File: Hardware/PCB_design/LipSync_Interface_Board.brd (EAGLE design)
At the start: 69.8 x 63.5 mm, 31 parts, among them T1 2N3906, U2 SF_MATE_RN42, U3 MPXV7002

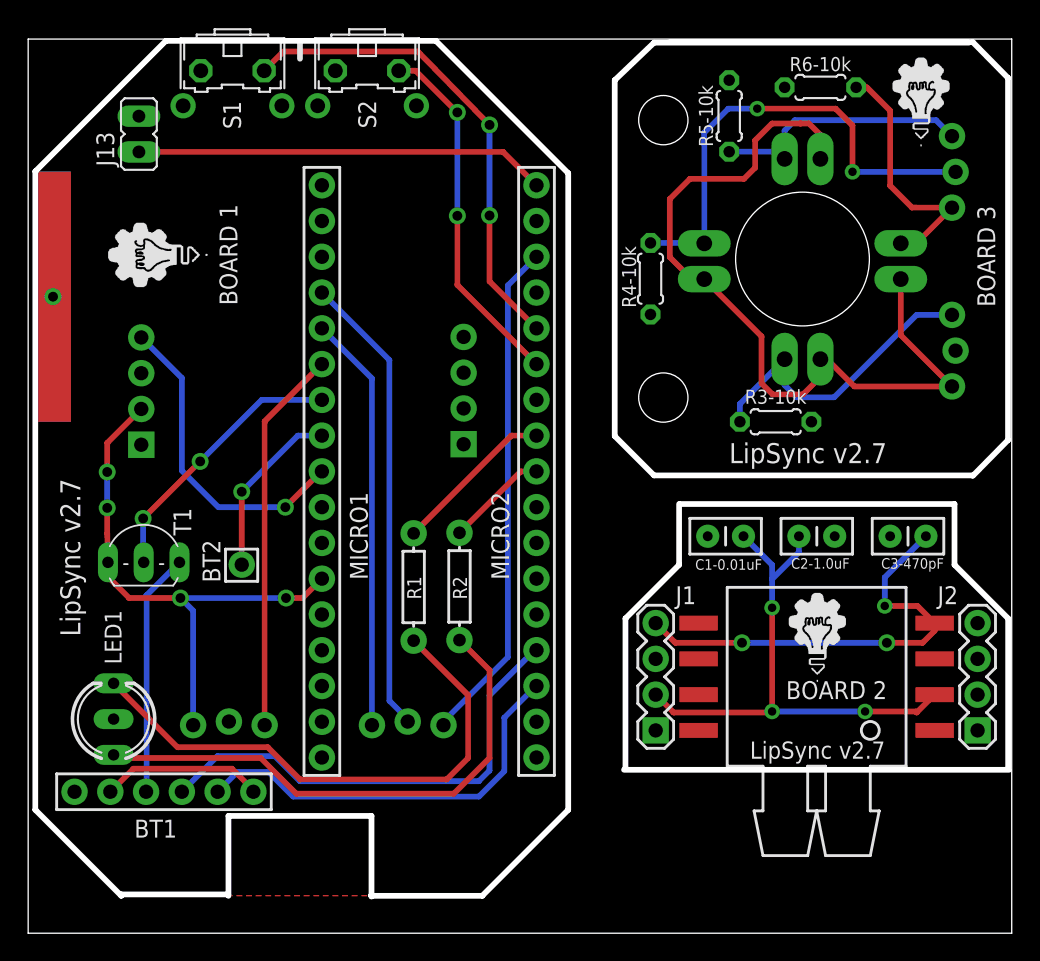
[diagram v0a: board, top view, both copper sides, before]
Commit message: Added PCB files Version 2.71 with updated MMC Logo.
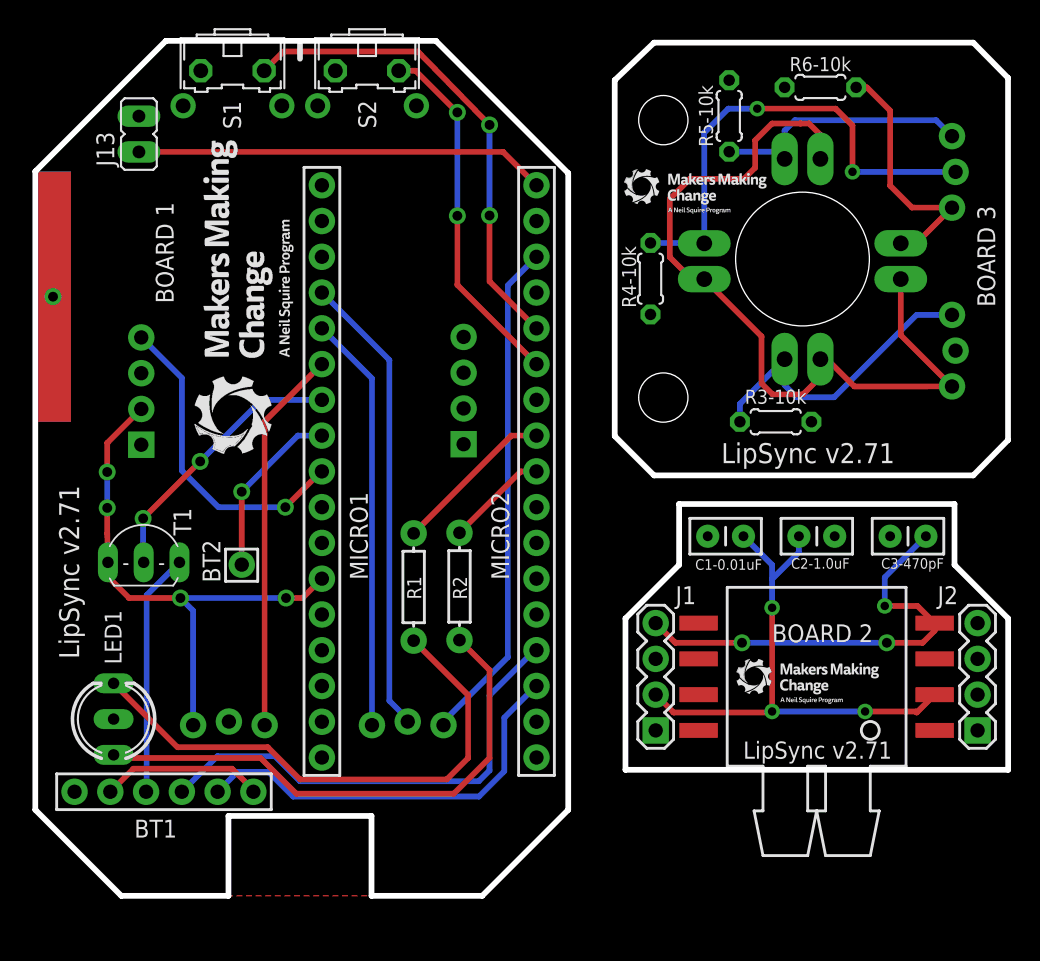
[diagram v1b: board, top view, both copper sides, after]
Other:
- board size 69.8 x 63.5 mm -> 69.1 x 60.7 mm
- board text added: "LipSync v2.71"
- board text removed: "LipSync v2.7"
